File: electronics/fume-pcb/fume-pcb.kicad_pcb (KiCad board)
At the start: 2 copper layers, 122.8 x 87.2 mm, 1 part

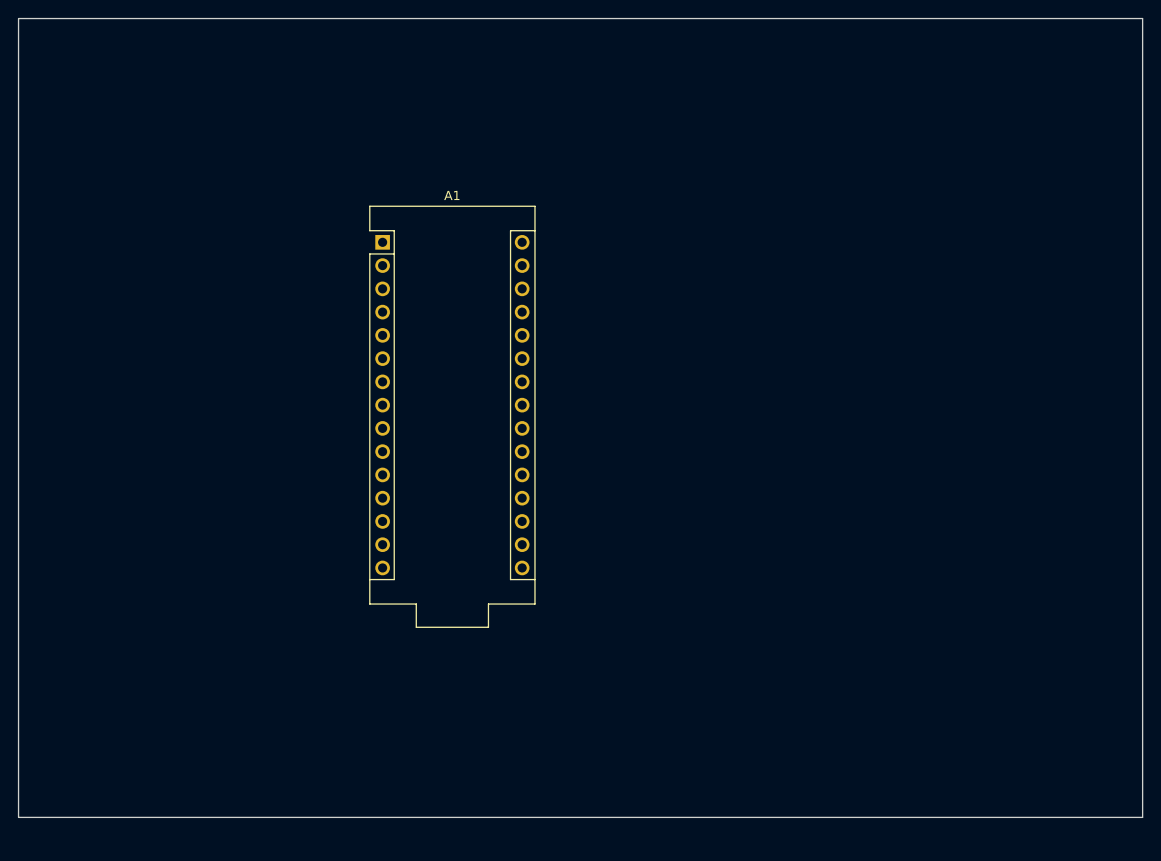
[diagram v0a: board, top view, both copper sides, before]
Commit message: Update
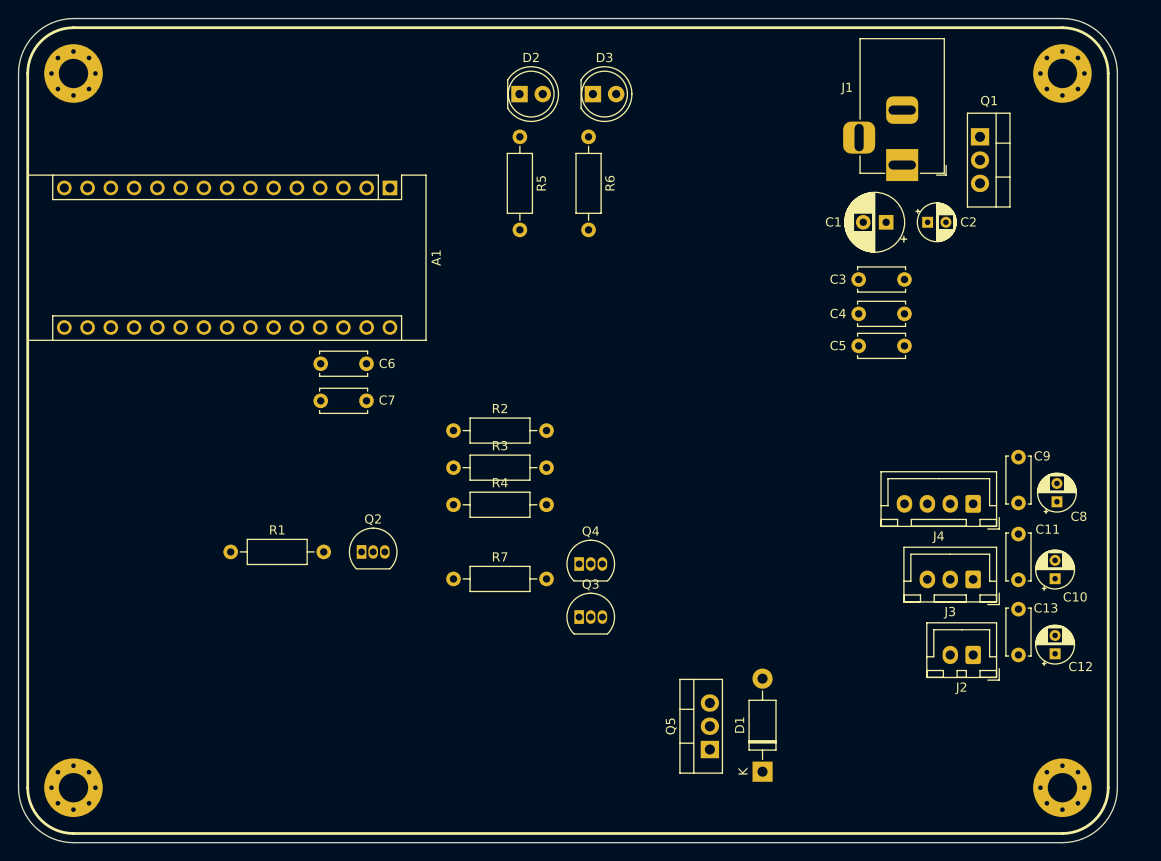
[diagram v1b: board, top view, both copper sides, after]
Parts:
- added C1: 220uF, Capacitor_THT:CP_Radial_D6.3mm_P2.50mm, F.Cu at (179.8, 72.2)
- added C10: 22uF, Capacitor_THT:CP_Radial_D4.0mm_P2.00mm, F.Cu at (198.2, 111.2)
- added C11: 0.1uF, Capacitor_THT:C_Disc_D5.0mm_W2.5mm_P5.00mm, F.Cu at (194.2, 111.3)
- added C12: 22uF, Capacitor_THT:CP_Radial_D4.0mm_P2.00mm, F.Cu at (198.2, 119.4)
- added C13: 0.1uF, Capacitor_THT:C_Disc_D5.0mm_W2.5mm_P5.00mm, F.Cu at (194.2, 119.5)
- added C2: 22uF, Capacitor_THT:CP_Radial_D4.0mm_P2.00mm, F.Cu at (184.3, 72.2)
- added C3: 10uF, Capacitor_THT:C_Disc_D5.0mm_W2.5mm_P5.00mm, F.Cu at (181.8, 78.5)
- added C4: 1uF, Capacitor_THT:C_Disc_D5.0mm_W2.5mm_P5.00mm, F.Cu at (181.8, 82.2)
- added C5: 0.1uF, Capacitor_THT:C_Disc_D5.0mm_W2.5mm_P5.00mm, F.Cu at (181.8, 85.8)
- added C6: 1uF, Capacitor_THT:C_Disc_D5.0mm_W2.5mm_P5.00mm, F.Cu at (118.0, 87.7)
- added C7: 0.1uF, Capacitor_THT:C_Disc_D5.0mm_W2.5mm_P5.00mm, F.Cu at (118.0, 91.8)
- added C8: 22uF, Capacitor_THT:CP_Radial_D4.0mm_P2.00mm, F.Cu at (198.4, 102.8)
- added C9: 0.1uF, Capacitor_THT:C_Disc_D5.0mm_W2.5mm_P5.00mm, F.Cu at (194.2, 102.9)
- added D1: 1N5819, Diode_THT:D_DO-41_SOD81_P10.16mm_Horizontal, F.Cu at (166.2, 132.2)
- added D2: BLUE, LED_THT:LED_D5.0mm, F.Cu at (139.7, 58.2)
- added D3: RED, LED_THT:LED_D5.0mm, F.Cu at (147.7, 58.2)
- added H1: MHole, MountingHole:MountingHole_3.2mm_M3_Pad_Via, F.Cu at (91.0, 56.0)
- added H2: MHole, MountingHole:MountingHole_3.2mm_M3_Pad_Via, F.Cu at (199.0, 56.0)
- added H3: MHole, MountingHole:MountingHole_3.2mm_M3_Pad_Via, F.Cu at (199.0, 134.0)
- added H4: MHole, MountingHole:MountingHole_3.2mm_M3_Pad_Via, F.Cu at (91.0, 134.0)
- added J1: PWR Conn, Connector_BarrelJack:BarrelJack_Horizontal, F.Cu at (181.5, 66.0)
- added J2: Conn_01x02, Connector_JST:JST_XH_B2B-XH-A_1x02_P2.50mm_Vertical, F.Cu at (189.2, 119.5)
- added J3: Conn_01x03, Connector_JST:JST_XH_B3B-XH-A_1x03_P2.50mm_Vertical, F.Cu at (189.2, 111.2)
- added J4: Conn_01x04, Connector_JST:JST_XH_B4B-XH-A_1x04_P2.50mm_Vertical, F.Cu at (189.2, 103.0)
- added Q1: STP12PF06, Package_TO_SOT_THT:TO-220-3_Vertical, F.Cu at (190.0, 62.9)
- added Q2: 2N3904, Package_TO_SOT_THT:TO-92_Inline, F.Cu at (122.5, 108.2)
- added Q3: 2N3906, Package_TO_SOT_THT:TO-92_Inline, F.Cu at (146.2, 115.4)
- added Q4: 2N3904, Package_TO_SOT_THT:TO-92_Inline, F.Cu at (146.2, 109.6)
- added Q5: IRFZ44N, Package_TO_SOT_THT:TO-220-3_Vertical, F.Cu at (160.5, 129.8)
- added R1: 1k, Resistor_THT:R_Axial_DIN0207_L6.3mm_D2.5mm_P10.16mm_Horizontal, F.Cu at (108.2, 108.2)
- added R2: 4.7k, Resistor_THT:R_Axial_DIN0207_L6.3mm_D2.5mm_P10.16mm_Horizontal, F.Cu at (132.5, 95.0)
- added R3: 2.2k, Resistor_THT:R_Axial_DIN0207_L6.3mm_D2.5mm_P10.16mm_Horizontal, F.Cu at (132.5, 99.0)
- added R4: 2.2k, Resistor_THT:R_Axial_DIN0207_L6.3mm_D2.5mm_P10.16mm_Horizontal, F.Cu at (132.5, 103.1)
- added R5: 1k, Resistor_THT:R_Axial_DIN0207_L6.3mm_D2.5mm_P10.16mm_Horizontal, F.Cu at (139.8, 62.9)
- added R6: 5.1k, Resistor_THT:R_Axial_DIN0207_L6.3mm_D2.5mm_P10.16mm_Horizontal, F.Cu at (147.2, 62.9)
- added R7: 4.7k, Resistor_THT:R_Axial_DIN0207_L6.3mm_D2.5mm_P10.16mm_Horizontal, F.Cu at (132.5, 111.2)
- moved A1 5.99 mm to (125.6, 68.5), turned to -90 degrees
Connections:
- A1 pad 12: unconnected-(A1-D9-Pad12) -> /PWM_FAN
- A1 pad 13: unconnected-(A1-D10-Pad13) -> /PWM_MOS
- A1 pad 19: unconnected-(A1-A0-Pad19) -> /REF_FAN
- A1 pad 5: unconnected-(A1-D2-Pad5) -> /ENC_FAN
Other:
- board size 122.8 x 87.2 mm -> 120 x 90 mm
